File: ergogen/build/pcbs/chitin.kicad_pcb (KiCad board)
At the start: 2 copper layers, 134 x 106.7 mm, 122 parts, among them J1 qwiik_jst

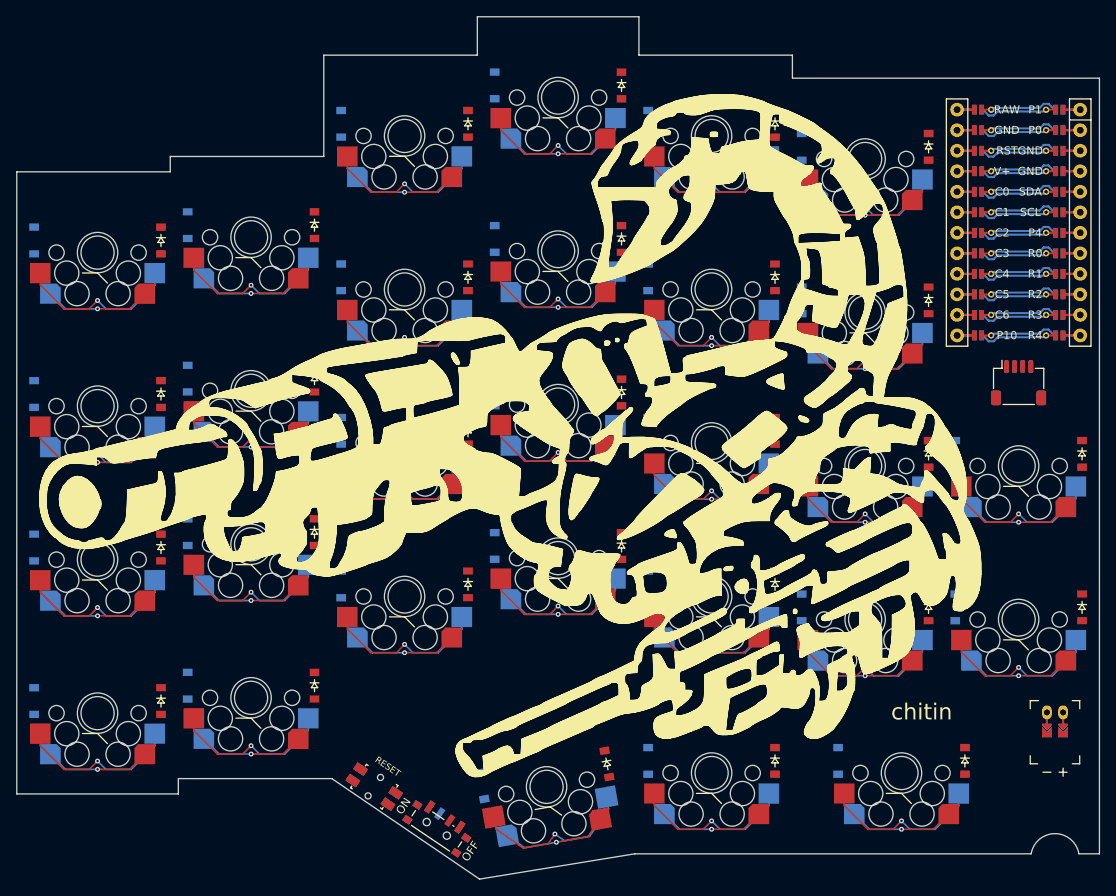
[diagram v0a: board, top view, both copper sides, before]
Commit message: Build
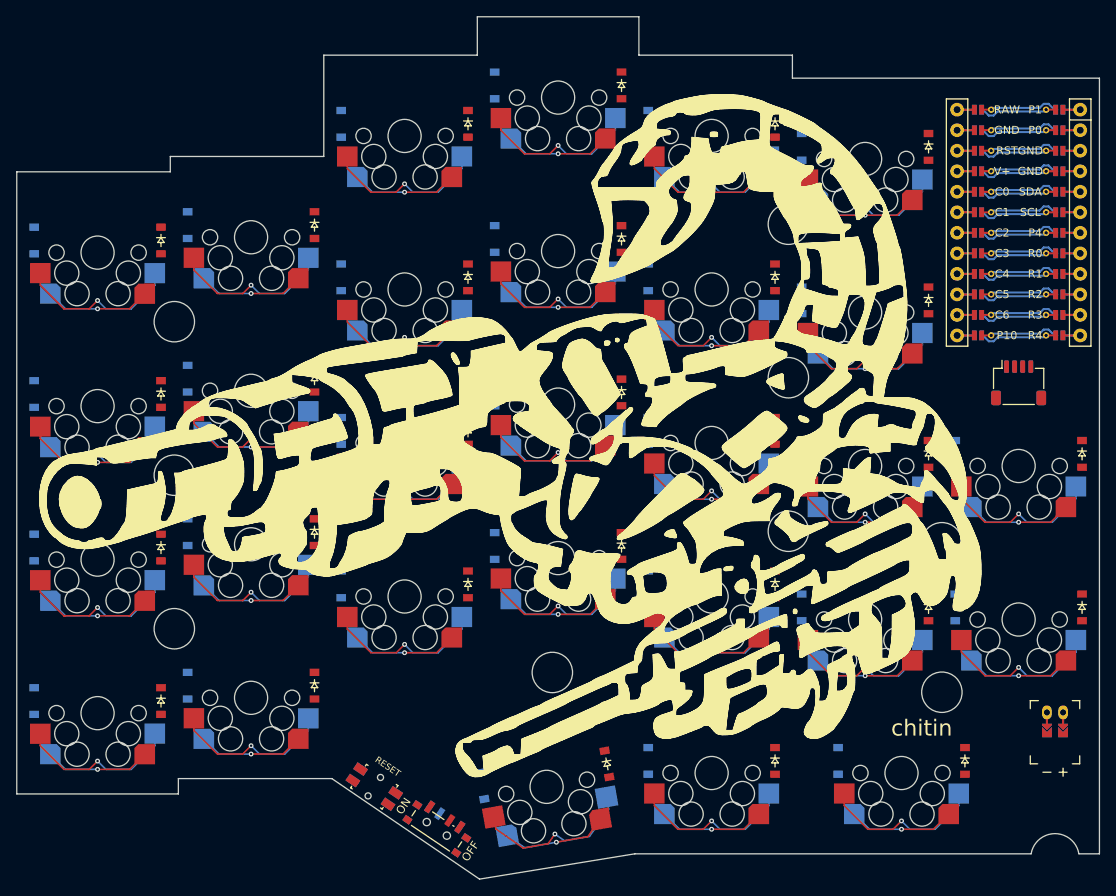
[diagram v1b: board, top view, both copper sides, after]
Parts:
- removed MH10, MH11, MH12, MH13, MH14, MH15, MH16, MH17, MH18, MH19, MH20, MH21, MH22, MH23, MH24, MH25, MH26, MH27, MH28, MH29: , ceoloide:mounting_hole_npth
- moved MH8 93.5 mm to (204.5, 128.9)
- moved MH5 88.6 mm to (185.5, 89.5)
- moved MH4 76.6 mm to (156.3, 145.0)
- moved MH6 69.6 mm to (185.5, 108.5)
- moved MH7 68.7 mm to (185.5, 127.5)
- moved MH9 67.5 mm to (204.5, 147.4)
- moved MH1 49.4 mm to (109.5, 101.5)
- moved MH3 29.1 mm to (109.5, 139.6)
- moved MH2 14.1 mm to (109.5, 120.5)
